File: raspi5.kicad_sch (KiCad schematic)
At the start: 6 parts, among them J1 GPIO, U1 FT24C256A

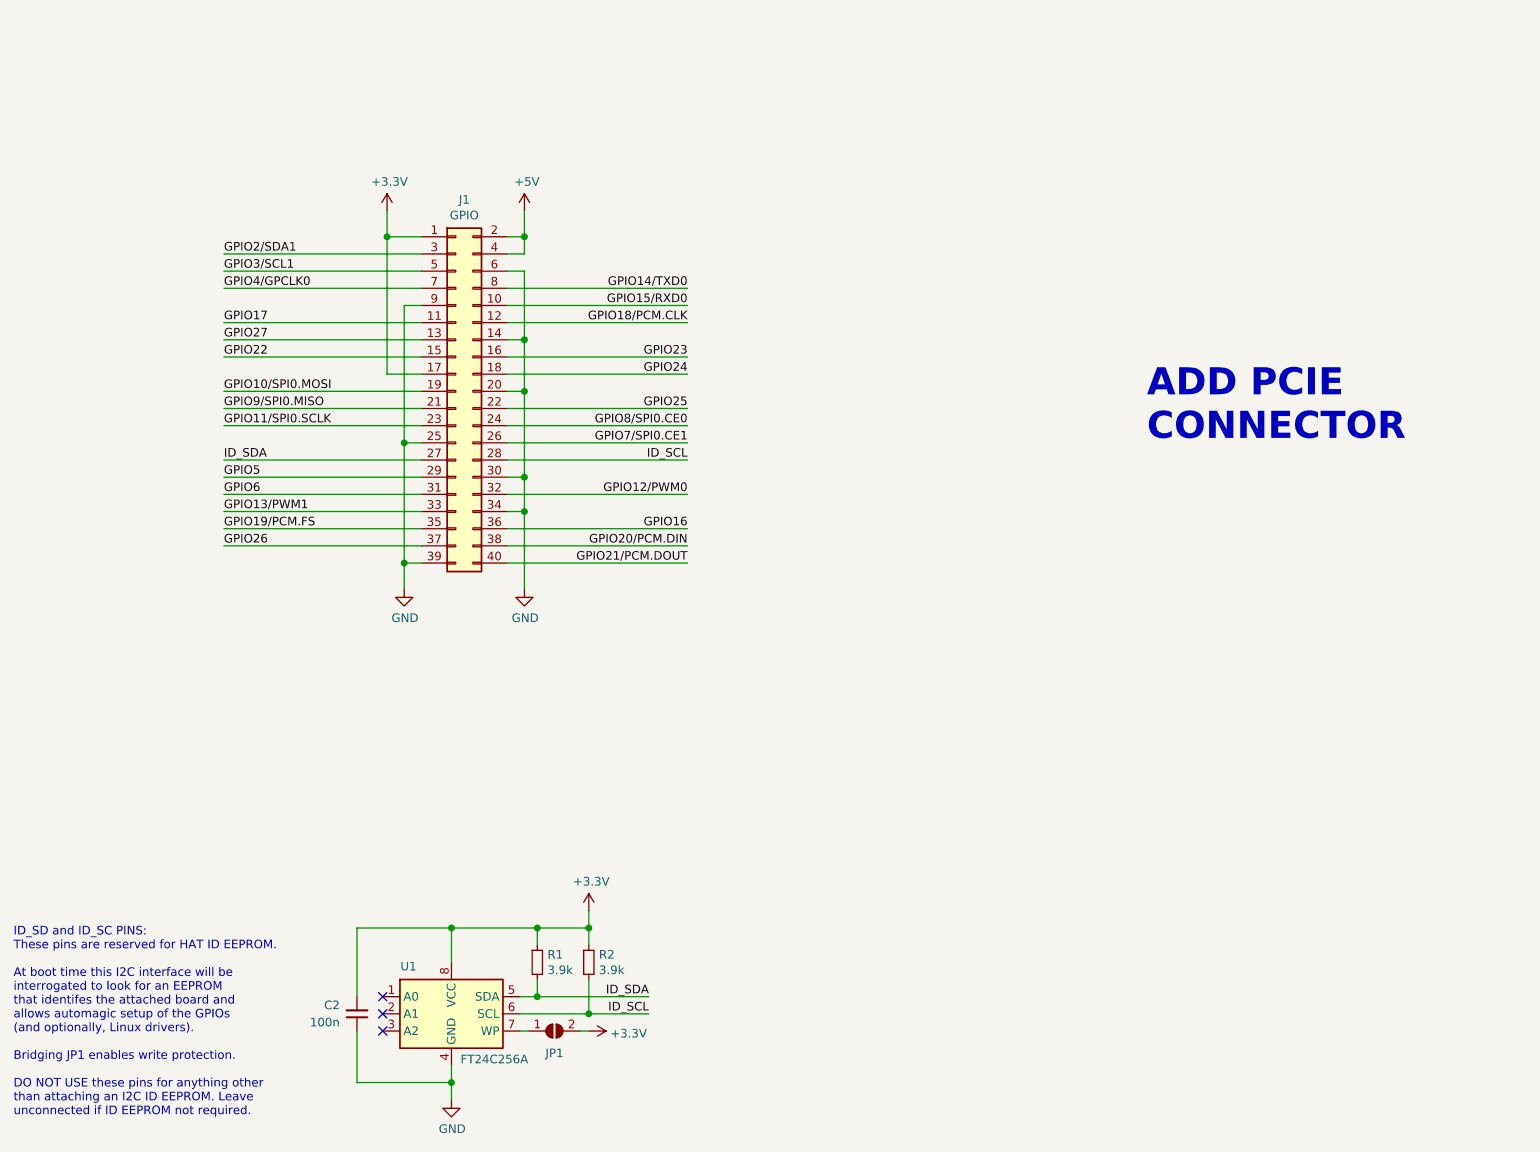
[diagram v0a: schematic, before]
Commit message: Schematic finished, starting layout
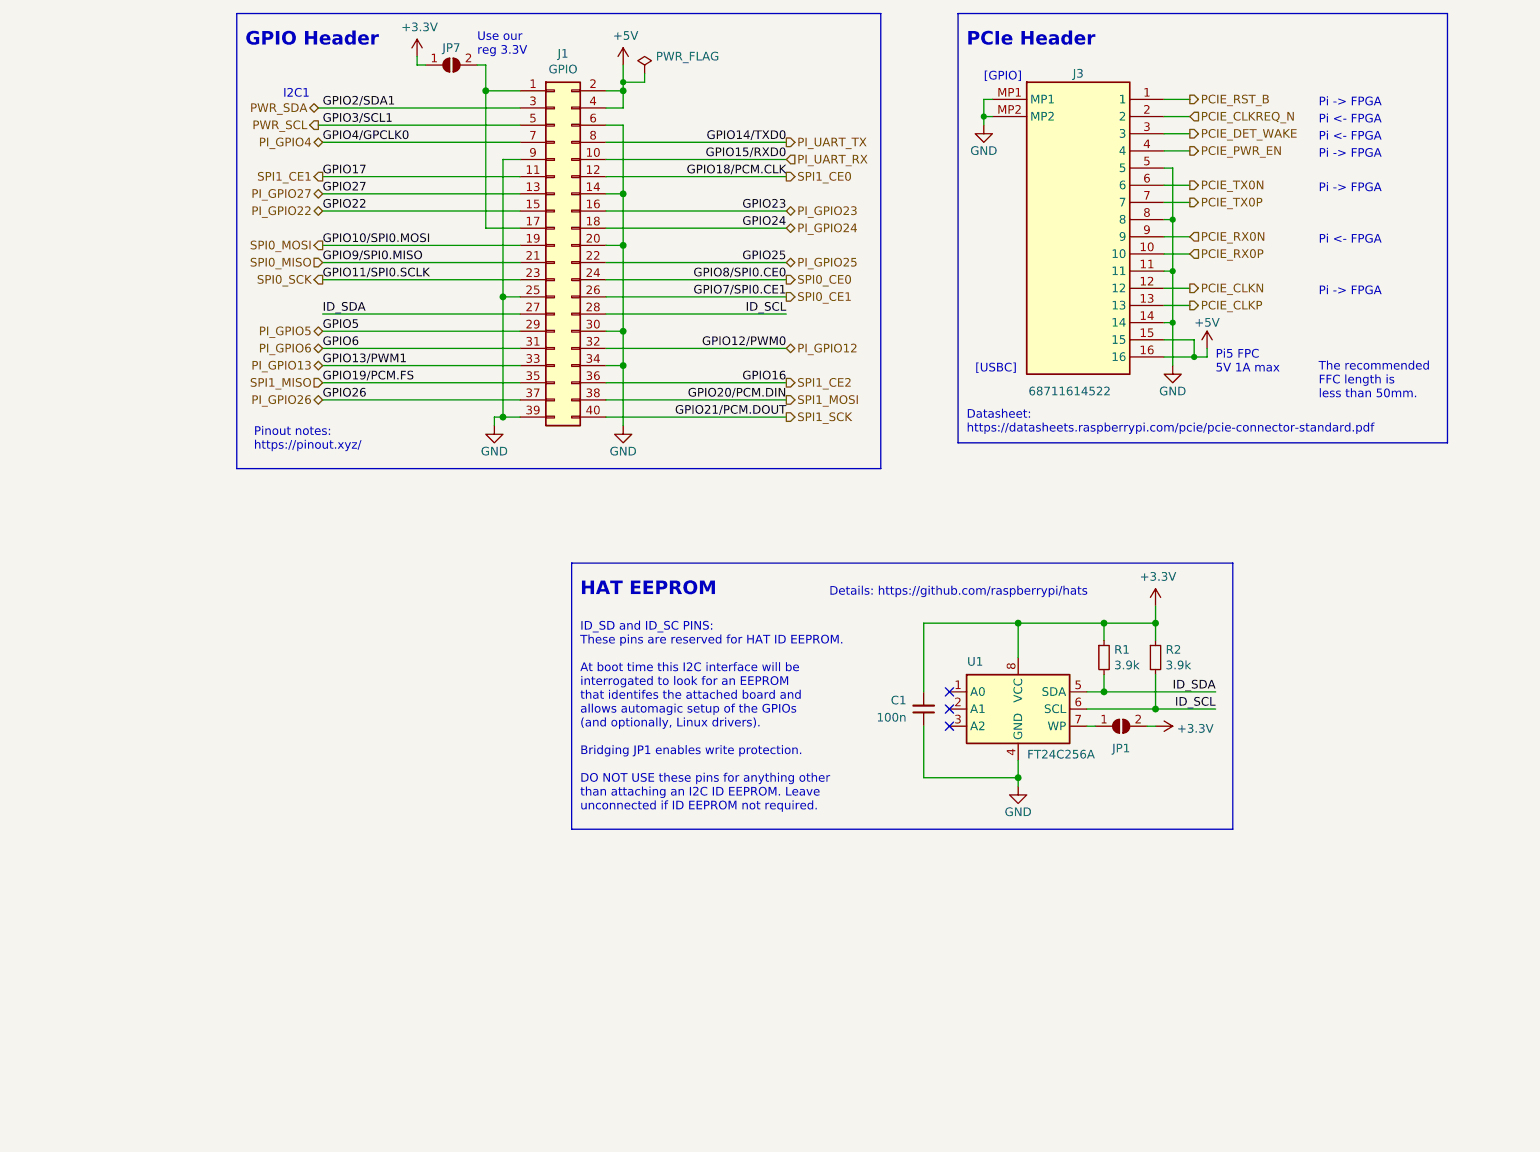
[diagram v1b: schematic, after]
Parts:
- added J3: 68711614522, 68711614522, symbol fpc:68711614522
- added JP7: ID_WP, Jumper:SolderJumper-2_P1.3mm_Open_TrianglePad1.0x1.5mm, symbol Jumper:SolderJumper_2_Open
- JP1: footprint (none) -> Jumper:SolderJumper-2_P1.3mm_Open_TrianglePad1.0x1.5mm
- R1, R2: footprint Resistor_SMD:R_0603_1608Metric_Pad0.98x0.95mm_HandSolder -> Resistor_SMD:R_0402_1005Metric_Pad0.72x0.64mm_HandSolder; LCSC C23018 -> (none)
- U1: footprint (none) -> Package_SO:MSOP-8_3x3mm_P0.65mm
- renumbered C2 to C1
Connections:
- net +3V3: now also JP7.1 (A); no longer J1.1 (Pin_1), J1.17 (Pin_17)
- net +5V: now also J3.15, J3.16
- net GND: now also J3.11, J3.14, J3.5, J3.8, J3.MP1, J3.MP2
- net GPIO10/SPI0.MOSI renamed SPI0_MOSI
- net GPIO11/SPI0.SCLK renamed SPI0_SCK
- net GPIO12/PWM0 renamed PI_GPIO12
- net GPIO13/PWM1 renamed PI_GPIO13
- net GPIO14/TXD0 renamed PI_UART_TX
- net GPIO15/RXD0 renamed PI_UART_RX
- net GPIO16 renamed SPI1_CE2
- net GPIO17 renamed SPI1_CE1
- net GPIO18/PCM.CLK renamed SPI1_CE0
- net GPIO19/PCM.FS renamed SPI1_MISO
- net GPIO20/PCM.DIN renamed SPI1_MOSI
- net GPIO21/PCM.DOUT renamed SPI1_SCK
- net GPIO22 renamed PI_GPIO22
- net GPIO23 renamed PI_GPIO23
- net GPIO24 renamed PI_GPIO24
- net GPIO25 renamed PI_GPIO25
- net GPIO26 renamed PI_GPIO26
- net GPIO27 renamed PI_GPIO27
- net GPIO2/SDA1 renamed PWR_SDA
- net GPIO3/SCL1 renamed PWR_SCL
- net GPIO4/GPCLK0 renamed PI_GPIO4
- net GPIO5 renamed PI_GPIO5
- net GPIO6 renamed PI_GPIO6
- net GPIO7/SPI0.CE1 renamed SPI0_CE1
- net GPIO8/SPI0.CE0 renamed SPI0_CE0
- net GPIO9/SPI0.MISO renamed SPI0_MISO
- new net: J1.1 (Pin_1), J1.17 (Pin_17), JP7.2 (B)
- new net PCIE_CLKN: J3.12
- new net PCIE_CLKP: J3.13
- new net PCIE_CLKREQ_N: J3.2
- new net PCIE_DET_WAKE: J3.3
- new net PCIE_PWR_EN: J3.4
- new net PCIE_RST_B: J3.1
- new net PCIE_RX0N: J3.9
- new net PCIE_RX0P: J3.10
- new net PCIE_TX0N: J3.6
- new net PCIE_TX0P: J3.7
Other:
- note added: "Datasheet: https://datasheets.raspberrypi.com/pcie/pcie-connector-standard.pdf"
- note added: "Details: https://github.com/raspberrypi/hats"
- note added: "GPIO Header"
- note added: "HAT EEPROM"
- note added: "I2C1"
- note added: "PCIe Header"
- note added: "Pi -> FPGA"
- note added: "Pi <- FPGA"
- note added: "Pi5 FPC 5V 1A max"
- note added: "Pinout notes: https://pinout.xyz/"
- note added: "The recommended FFC length is less than 50mm."
- note added: "Use our reg 3.3V"
- note added: "[GPIO]"
- note added: "[USBC]"
- note removed: "ADD PCIE CONNECTOR"
- title: Raspberry Pi 5 Connections -> FPGA Power
- moved on the sheet: C1, J1, JP1, R1, R2, U1
